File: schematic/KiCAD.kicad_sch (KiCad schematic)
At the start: 7 parts, among them J1 Raspberry_Pi_4, U1 NUCLEO-F401RE, U2 ACS712xLCTR-05B, U3 ACS712xLCTR-05B, U4 ACS712xLCTR-05B, U5 L298N

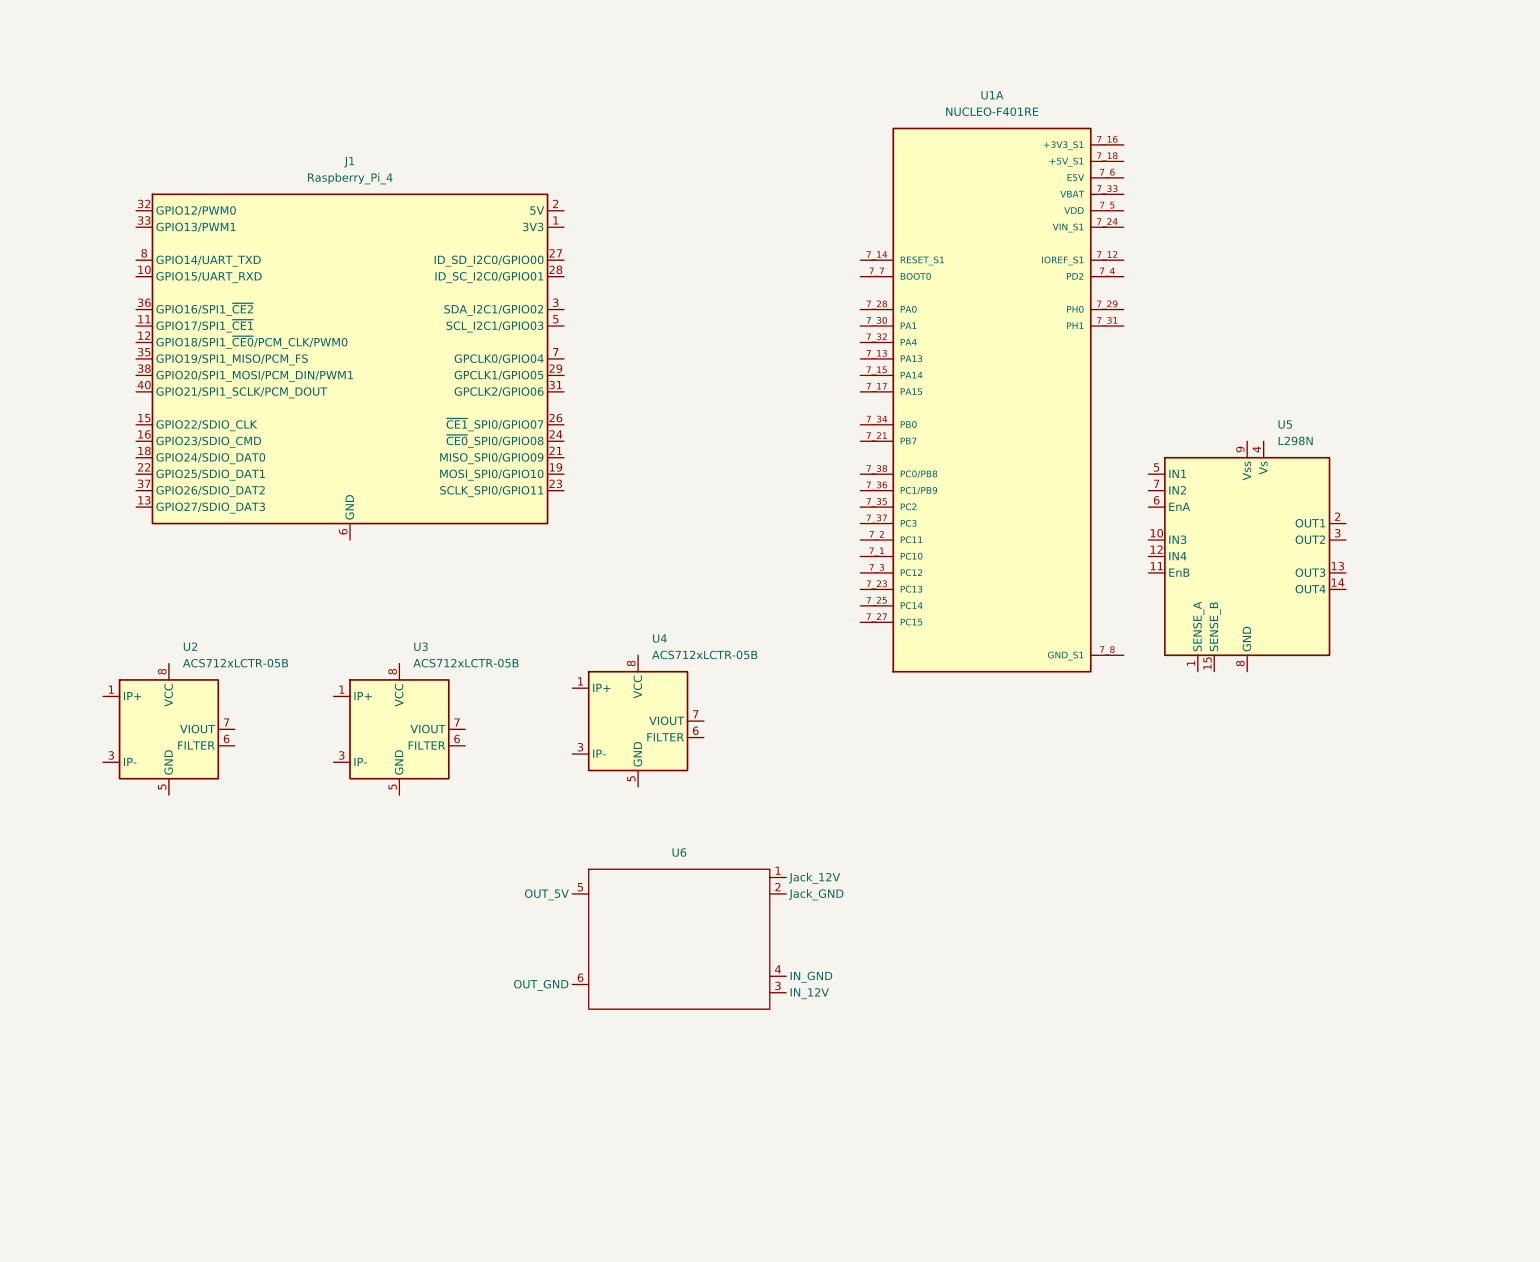
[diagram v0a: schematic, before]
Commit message: new schematic
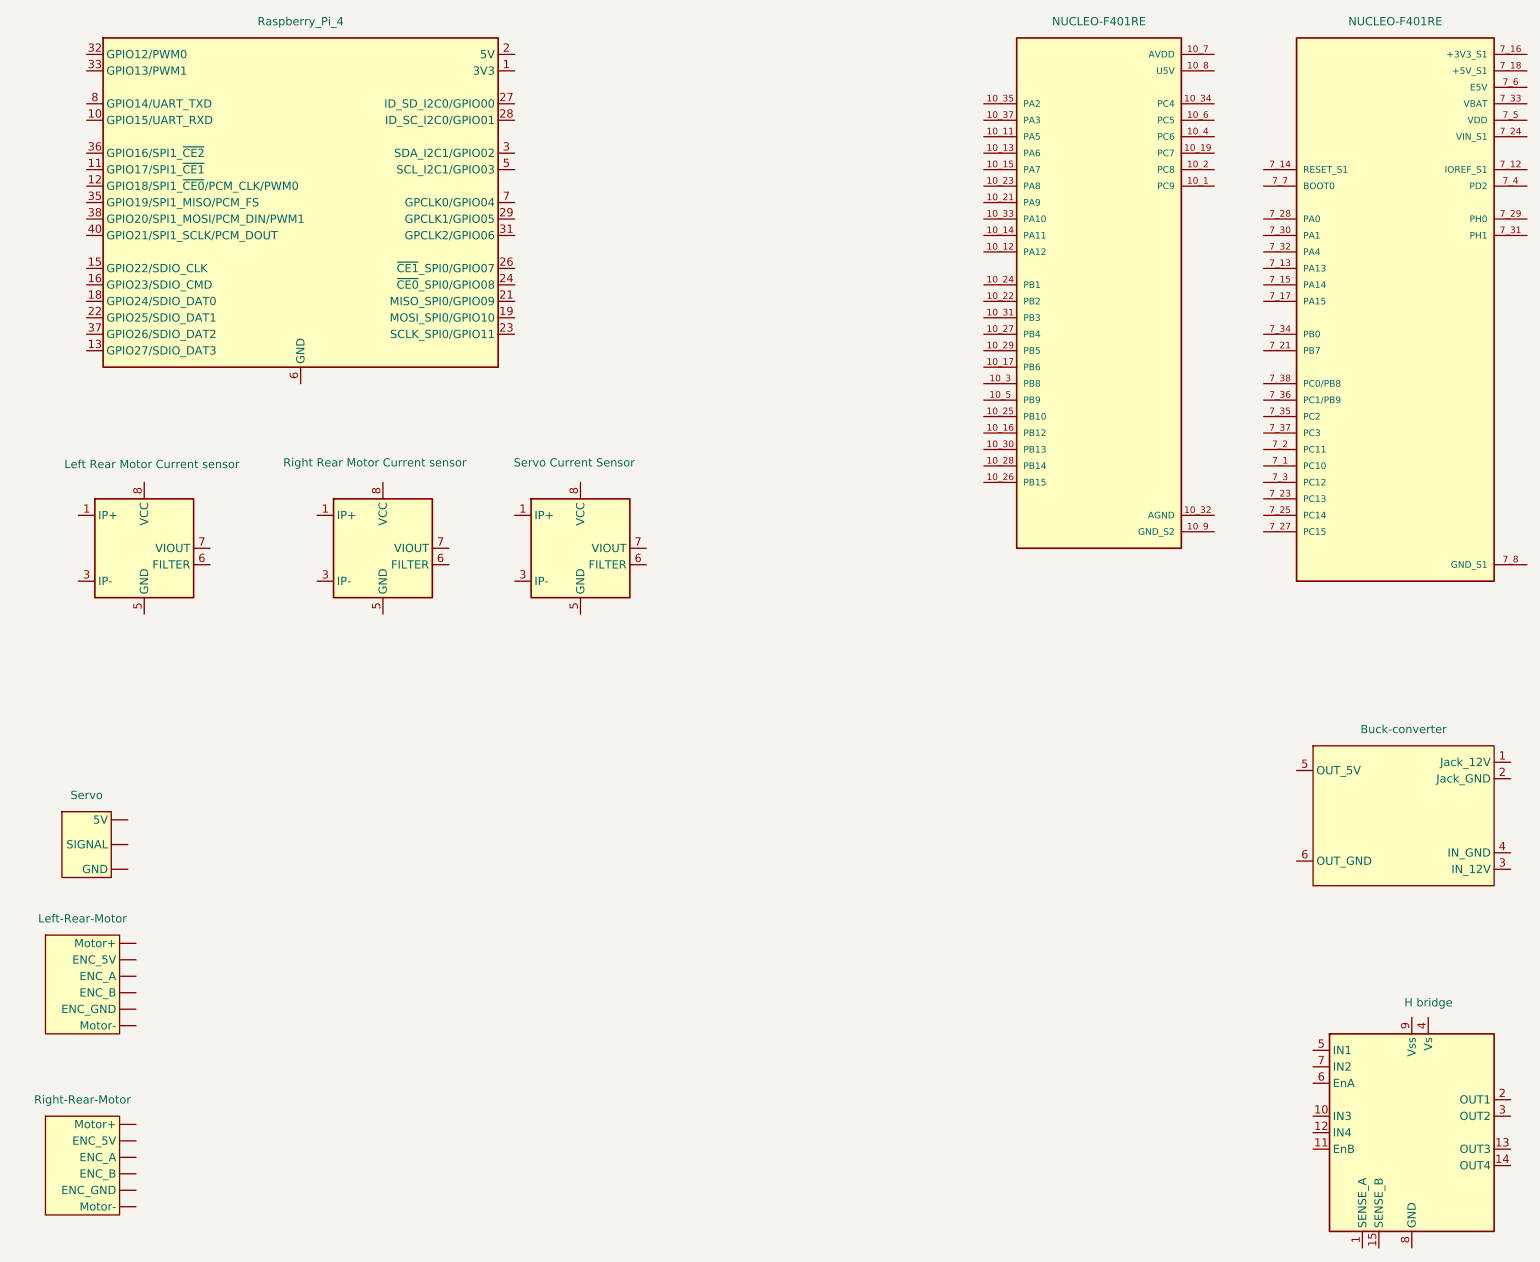
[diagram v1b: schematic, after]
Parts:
- removed U6: (no value), Package_DFN_QFN:WDFN-10-1EP_3x3mm_P0.5mm_EP1.8x2.5mm, symbol Lab2_Modules:HW688_Buck
- added Buck-converter: (no value), symbol Lab2_Modules:HW688_Buck
- added Left-Rear-Motor, Right-Rear-Motor: (no value), symbol Lab2_Modules:Motor_With_Encoder
- added Servo: (no value), symbol Lab2_Modules:Servo
- U2: value ACS712xLCTR-05B -> Left Rear Motor Current sensor
- U3: value ACS712xLCTR-05B -> Right Rear Motor Current sensor
- U4: value ACS712xLCTR-05B -> Servo Current Sensor
- U5: value L298N -> H bridge
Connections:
- new net GND_S2: U1.10_20 (GND_S2), U1.10_9 (GND_S2)
